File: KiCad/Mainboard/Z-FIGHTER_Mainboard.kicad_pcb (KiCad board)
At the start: 2 copper layers, 100 x 150 mm, 52 parts, among them IC1 Z80SIO, J1 DB9_Male_MountingHoles, J2 DB9_Male_MountingHoles, J3 USB_B, J4 Conn_02x13_Odd_Even, J5 Conn_Parallel_User, J6 Conn_PATA, J7 Conn_02x03_Odd_Even, SW1 SW_Push, SW2 SW_DIP_x03, U1 AS6C4008-55PCN, U10 DS1233, U2 Z80CPU, U3 82C55A, U4 SST39SF040, U5 MAX203, U6 MAX203, U7 ATF22V10CZ-15PI, U8 74HC00, U9 82C55A, X1 Z80/SIO Ch.A Clock, X2 SIO Ch.B Clock

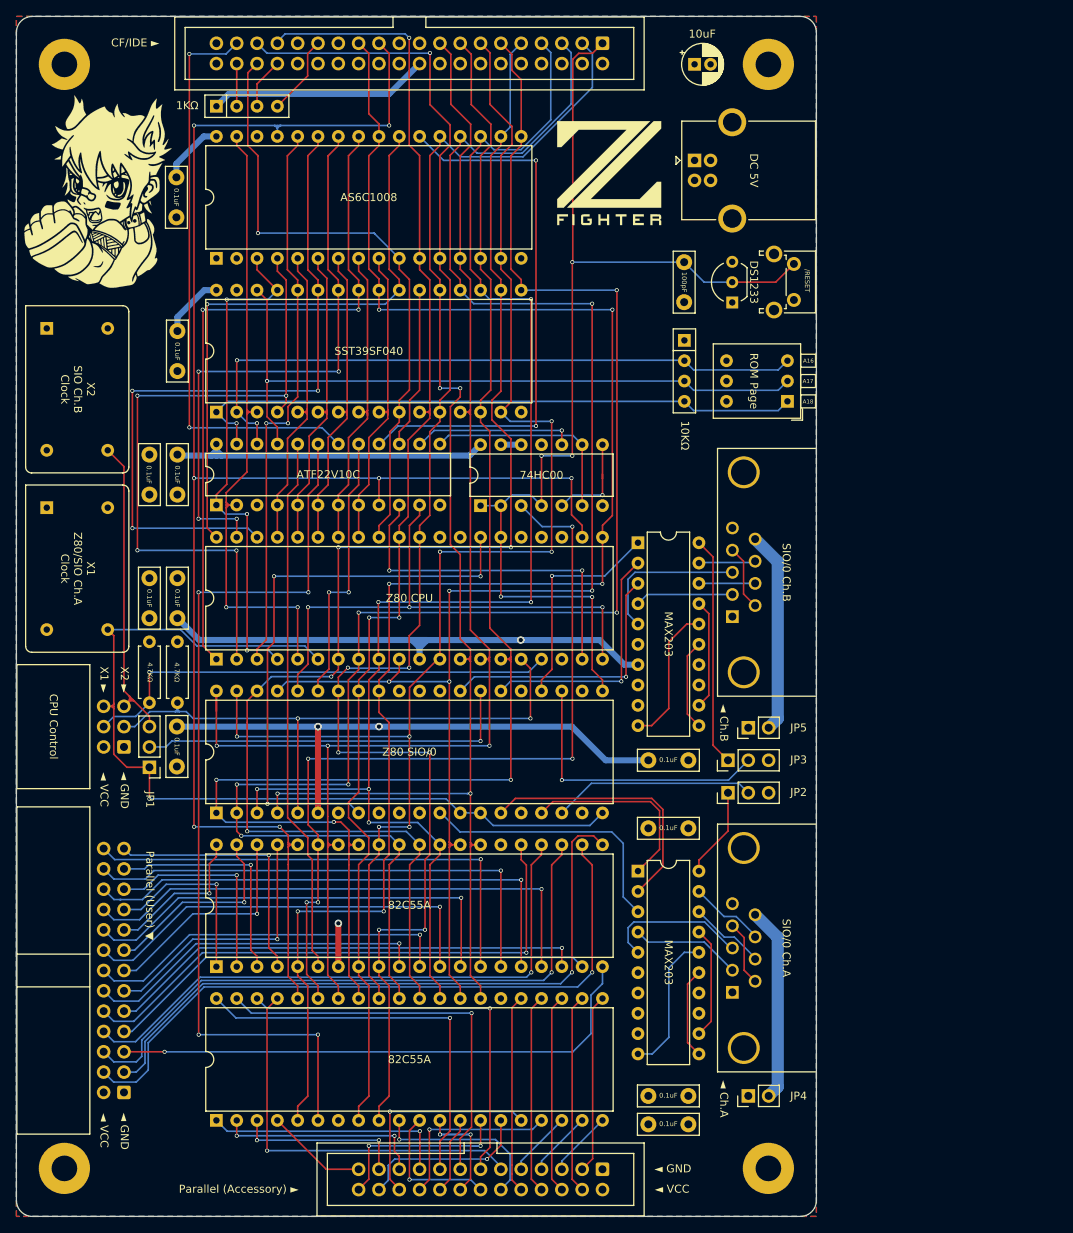
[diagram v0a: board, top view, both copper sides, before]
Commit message: Board illustrations
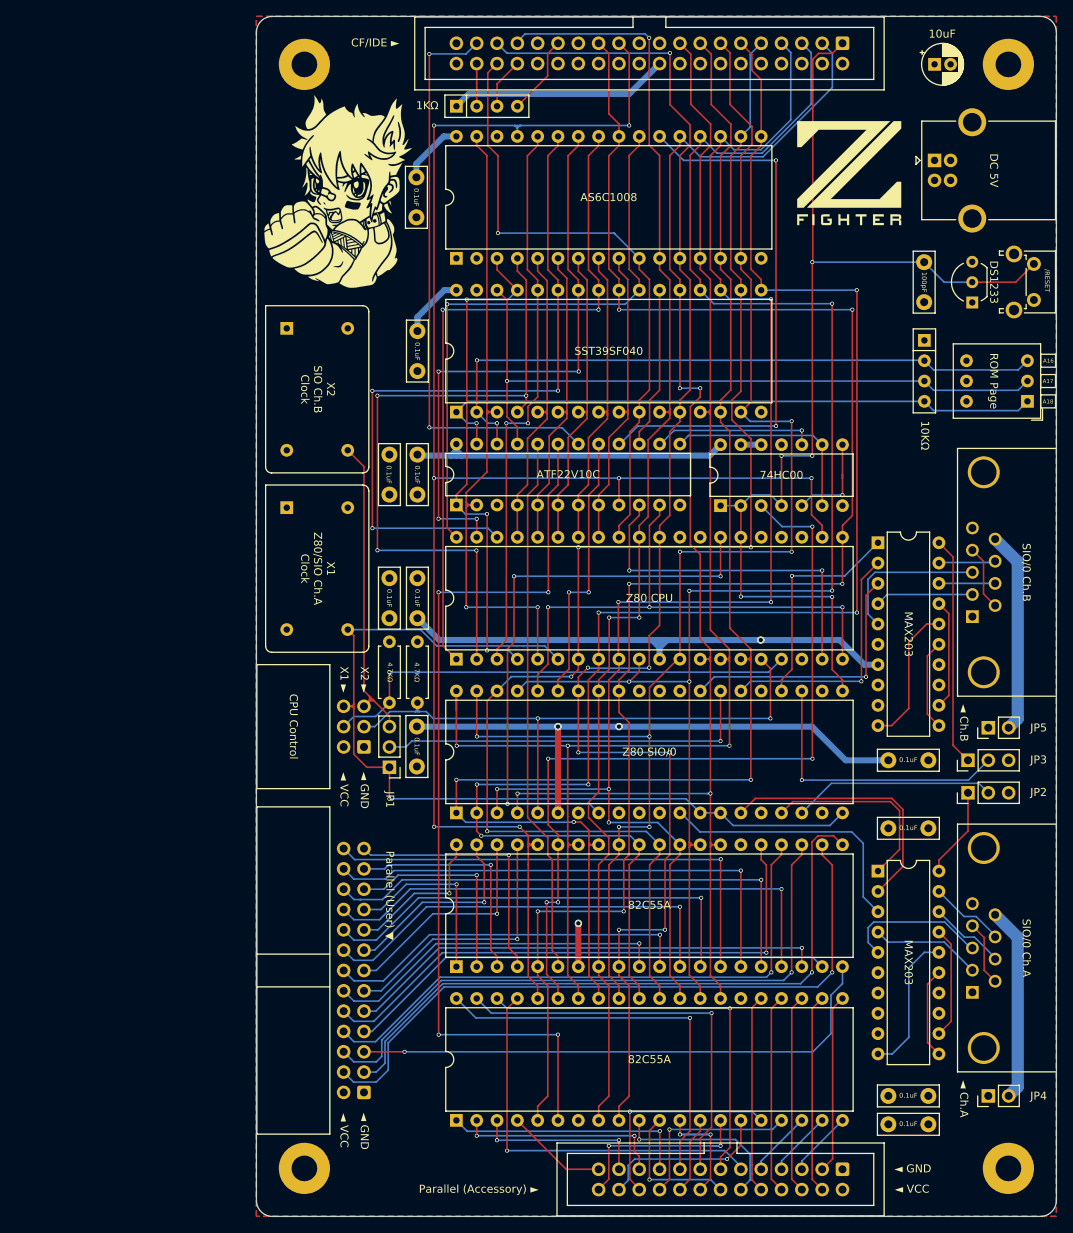
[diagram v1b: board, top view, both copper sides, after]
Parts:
- moved C2 30.0 mm to (151.4, 62.7)
- moved J1 30.0 mm to (157.4, 149.0)
- moved J2 30.0 mm to (157.4, 102.0)
- moved RN2 30.0 mm to (151.4, 67.5)
- moved C3 30.0 mm to (84.5, 102.2)
- moved C6 30.0 mm to (88.0, 66.3)
- moved C7 30.0 mm to (88.0, 81.8)
- moved C8 30.0 mm to (88.0, 102.2)
- moved C9 30.0 mm to (84.5, 81.8)
- moved JP1 30.0 mm to (84.5, 120.9)
- moved R1 30.0 mm to (88.0, 105.2)
- moved R2 30.0 mm to (84.5, 105.2)
- moved C1 30.0 mm to (152.7, 33.0)
- moved C10 30.0 mm to (146.9, 161.9)
- moved C11 30.0 mm to (88.0, 115.8)
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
